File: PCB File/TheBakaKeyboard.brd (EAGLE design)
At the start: 48.3 x 48.3 mm, 7 parts

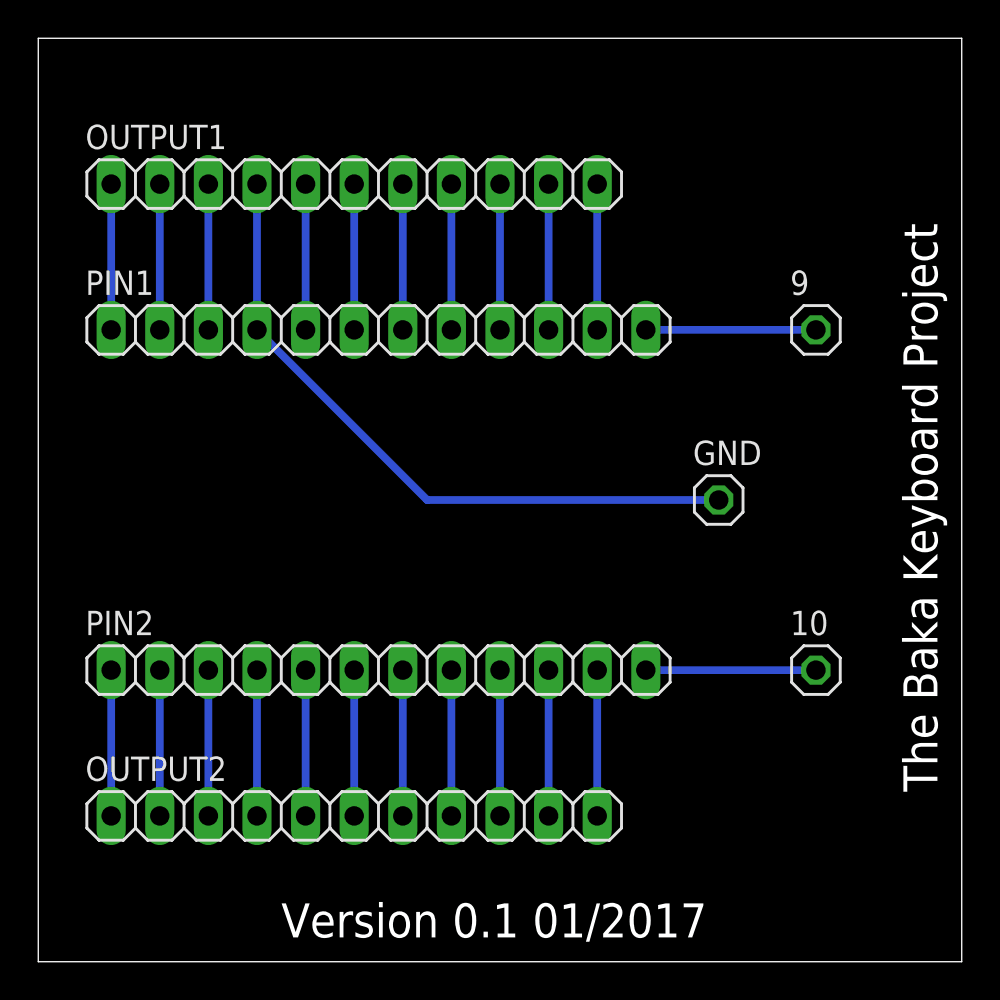
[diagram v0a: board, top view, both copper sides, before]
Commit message: update PCB and Model Design
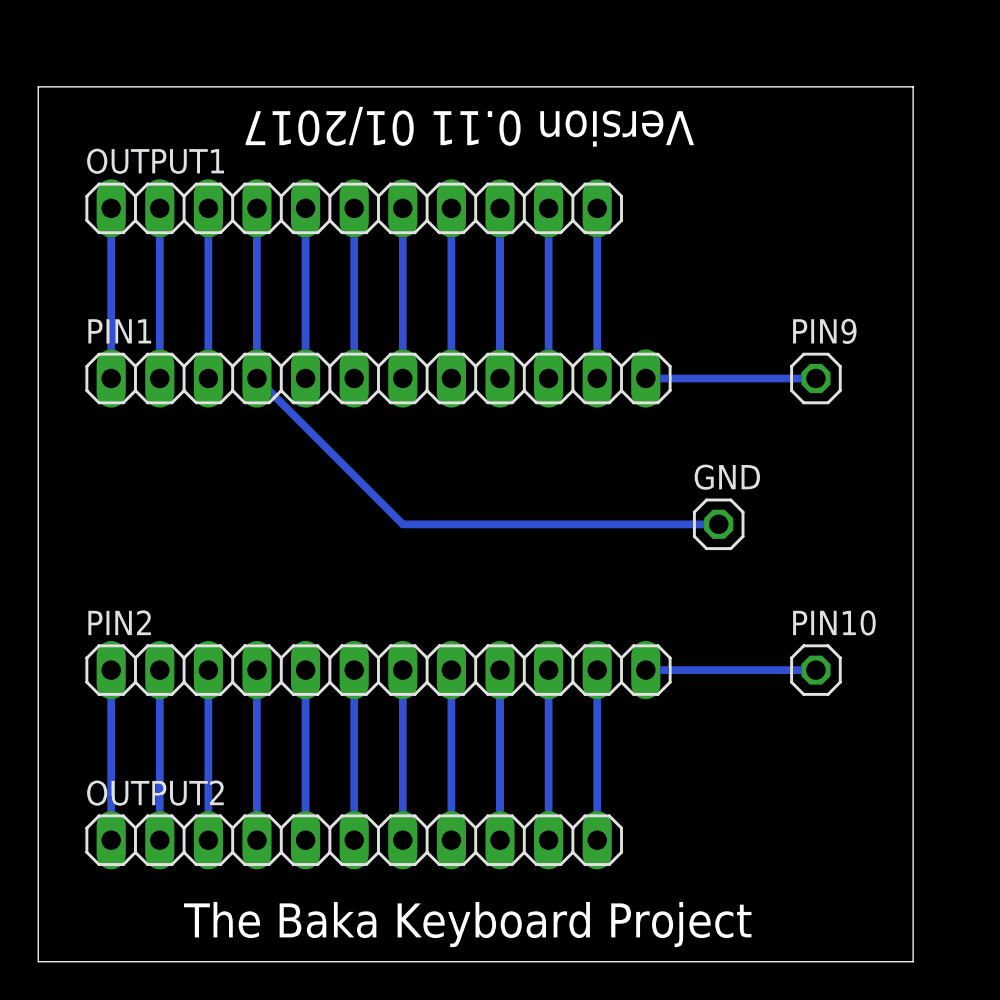
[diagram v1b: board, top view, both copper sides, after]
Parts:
- removed 9: (no value), pinhead:1X01
- added PIN9: (no value), pinhead:1X01
- moved PIN1 2.54 mm to (17.8, 30.5)
- moved OUTPUT1 1.27 mm to (16.5, 39.4)
- moved OUTPUT2 1.27 mm to (16.5, 6.35)
- moved GND 1.27 mm to (35.6, 22.9)
- renumbered 10 to PIN10
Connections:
- removed net S$22: OUTPUT1.2, PIN1.2
- new net S$3: OUTPUT1.3, PIN1.3
- net PIN9: now also PIN9.1; no longer 9.1
- net S$10: now also OUTPUT1.10, PIN1.10; no longer OUTPUT1.11, PIN1.11
- net S$11: now also OUTPUT1.11, PIN1.11; no longer OUTPUT2.11, PIN2.11
- net S$12: now also OUTPUT2.2, PIN2.2; no longer OUTPUT2.10, PIN2.10
- net S$13: now also OUTPUT2.3, PIN2.3; no longer OUTPUT2.9, PIN2.9
- net S$14: now also OUTPUT2.4, PIN2.4; no longer OUTPUT2.8, PIN2.8
- net S$15: now also OUTPUT2.5, PIN2.5; no longer OUTPUT2.7, PIN2.7
- net S$17: now also OUTPUT2.7, PIN2.7; no longer OUTPUT2.5, PIN2.5
- net S$18: now also OUTPUT2.8, PIN2.8; no longer OUTPUT2.4, PIN2.4
- net S$19: now also OUTPUT2.9, PIN2.9; no longer OUTPUT2.3, PIN2.3
- net S$2: now also OUTPUT1.2, PIN1.2; no longer OUTPUT1.3, PIN1.3
- net S$20: now also OUTPUT2.10, PIN2.10; no longer OUTPUT2.2, PIN2.2
- net S$21: now also OUTPUT2.11, PIN2.11; no longer OUTPUT2.1, PIN2.1
- net S$4: now also OUTPUT2.1, PIN2.1; no longer OUTPUT1.5, PIN1.5
- net S$5: now also OUTPUT1.5, PIN1.5; no longer OUTPUT1.6, PIN1.6
- net S$6: now also OUTPUT1.6, PIN1.6; no longer OUTPUT1.7, PIN1.7
- net S$7: now also OUTPUT1.7, PIN1.7; no longer OUTPUT1.8, PIN1.8
- net S$8: now also OUTPUT1.8, PIN1.8; no longer OUTPUT1.9, PIN1.9
- net S$9: now also OUTPUT1.9, PIN1.9; no longer OUTPUT1.10, PIN1.10
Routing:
- net S$3: track 0.00 -> 8.89 mm
- net S$22: track 7.62 -> 0.00 mm
- net S$4: track 7.62 -> 8.89 mm
- net S$21: track 7.62 -> 8.89 mm
- net S$20: track 7.62 -> 8.89 mm
- net S$19: track 7.62 -> 8.89 mm
- net S$18: track 7.62 -> 8.89 mm
- net S$17: track 7.62 -> 8.89 mm
- net S$16: track 7.62 -> 8.89 mm
- net S$15: track 7.62 -> 8.89 mm
- net S$14: track 7.62 -> 8.89 mm
- net S$13: track 7.62 -> 8.89 mm
- net S$12: track 7.62 -> 8.89 mm
- net S$9: track 7.62 -> 8.89 mm
- net S$8: track 7.62 -> 8.89 mm
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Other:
- board size 48.3 x 48.3 mm -> 45.7 x 45.7 mm
- board text added: "Version 0.11 01/2017"
- board text removed: "Version 0.1 01/2017"
